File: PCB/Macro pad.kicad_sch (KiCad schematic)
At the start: 11 parts, among them J1 Conn_01x04, SW1 SW_Push, SW2 SW_Push, SW3 SW_Push, SW4 SW_Push, SW5 SW_Push, SW6 SW_Push, SW9 RotaryEncoder_Switch, U1 XIAO-RP2040-DIP

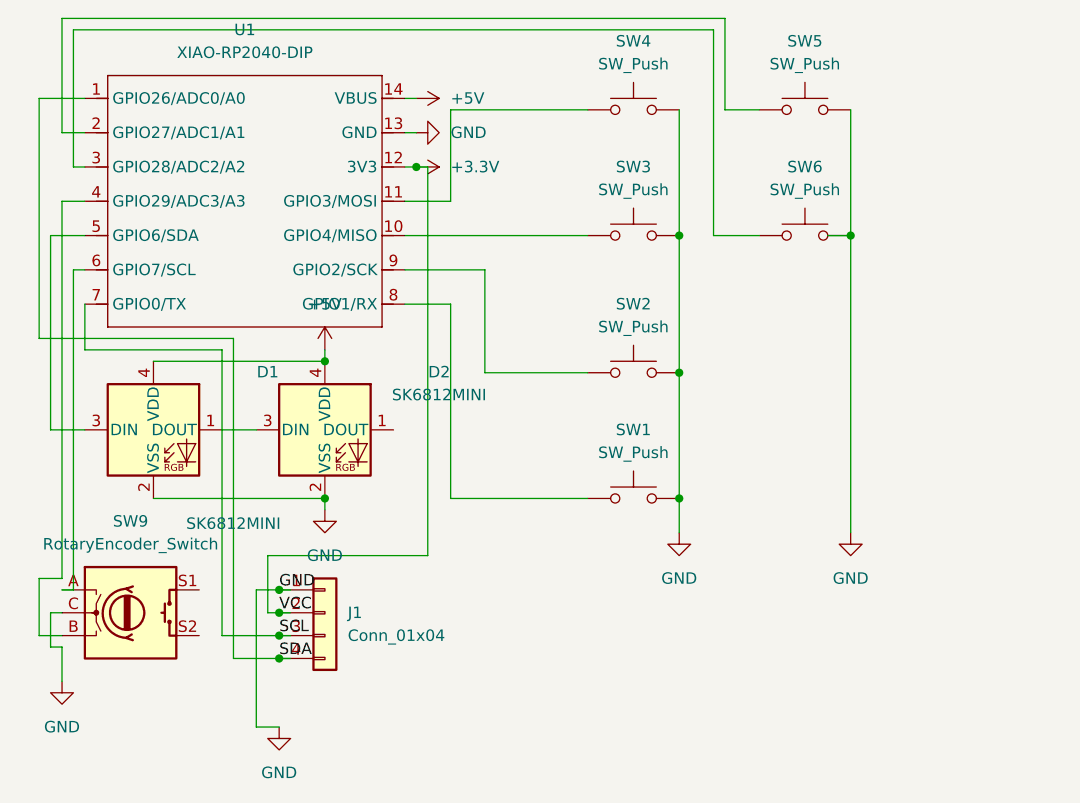
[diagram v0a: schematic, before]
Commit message: Add files via upload
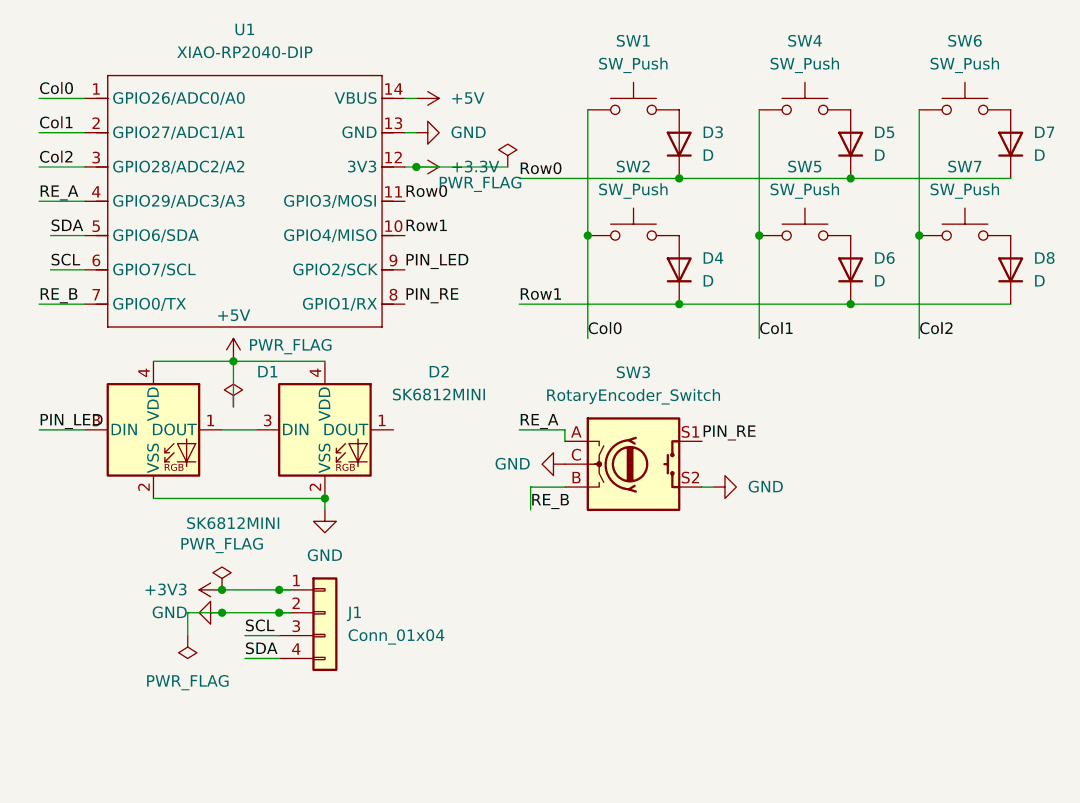
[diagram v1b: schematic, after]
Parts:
- added D3, D4, D5, D6, D7, D8: D, Diode_THT:D_DO-35_SOD27_P7.62mm_Horizontal, symbol Device:D
- renumbered SW4 to SW1, SW3 to SW2, SW9 to SW3, SW5 to SW4, SW6 to SW5, SW1 to SW6, SW2 to SW7
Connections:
- net +3.3V: no longer J1.2 (Pin_2)
- net GND: now also J1.2 (Pin_2), SW3.S2; no longer J1.1 (Pin_1), SW1.2, SW2.2, SW4.2, SW5.2, SW6.2, SW7.2
- net SCL: now also U1.6 (GPIO7/SCL); no longer U1.7 (GPIO0/TX)
- net SDA: now also U1.5 (GPIO6/SDA); no longer U1.1 (GPIO26/ADC0/A0)
- net RE_A: now reaches SW3.A
- net RE_A: now also U1.4 (GPIO29/ADC3/A3); no longer U1.6 (GPIO7/SCL)
- net RE_B: now reaches SW3.B
- net RE_B: now also U1.7 (GPIO0/TX); no longer U1.4 (GPIO29/ADC3/A3)
- net PIN_RE: now reaches SW3.S1
- net PIN_RE: now also U1.8 (GPIO1/RX)
- net PIN_LED: now reaches D1.3 (DIN)
- net PIN_LED: now also U1.9 (GPIO2/SCK); no longer U1.5 (GPIO6/SDA)
- net Col0: now reaches SW2.1
- net Col0: now also SW1.1, U1.1 (GPIO26/ADC0/A0); no longer U1.10 (GPIO4/MISO)
- net Row0: now reaches U1.11 (GPIO3/MOSI)
- net Row0: now also D3.1 (K), D5.1 (K), D7.1 (K); no longer SW1.1
- net Col2: now reaches SW6.1
- net Col2: now also SW7.1, U1.3 (GPIO28/ADC2/A2); no longer U1.8 (GPIO1/RX)
- net Col1: now reaches SW4.1, U1.2 (GPIO27/ADC1/A1)
- net Col1: now also SW5.1
- new net: D4.2 (A), SW2.2
- new net: D3.2 (A), SW1.2
- new net: D7.2 (A), SW6.2
- new net: D8.2 (A), SW7.2
- new net: D5.2 (A), SW4.2
- new net: D6.2 (A), SW5.2
- new net +3V3: J1.1 (Pin_1)
- new net Row1: D4.1 (K), D6.1 (K), D8.1 (K), U1.10 (GPIO4/MISO)
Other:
- moved on the sheet: SW3, SW6, SW7
